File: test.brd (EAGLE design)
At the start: 101.6 x 53.3 mm, 60 parts, among them IC2 ATMEGA1280-16AU, IC4 MC33269D-5.0, IC6 FT232RL, IC7 LM358D, Q2 16MHz, T1 NDT2955, X2 DC21MMX

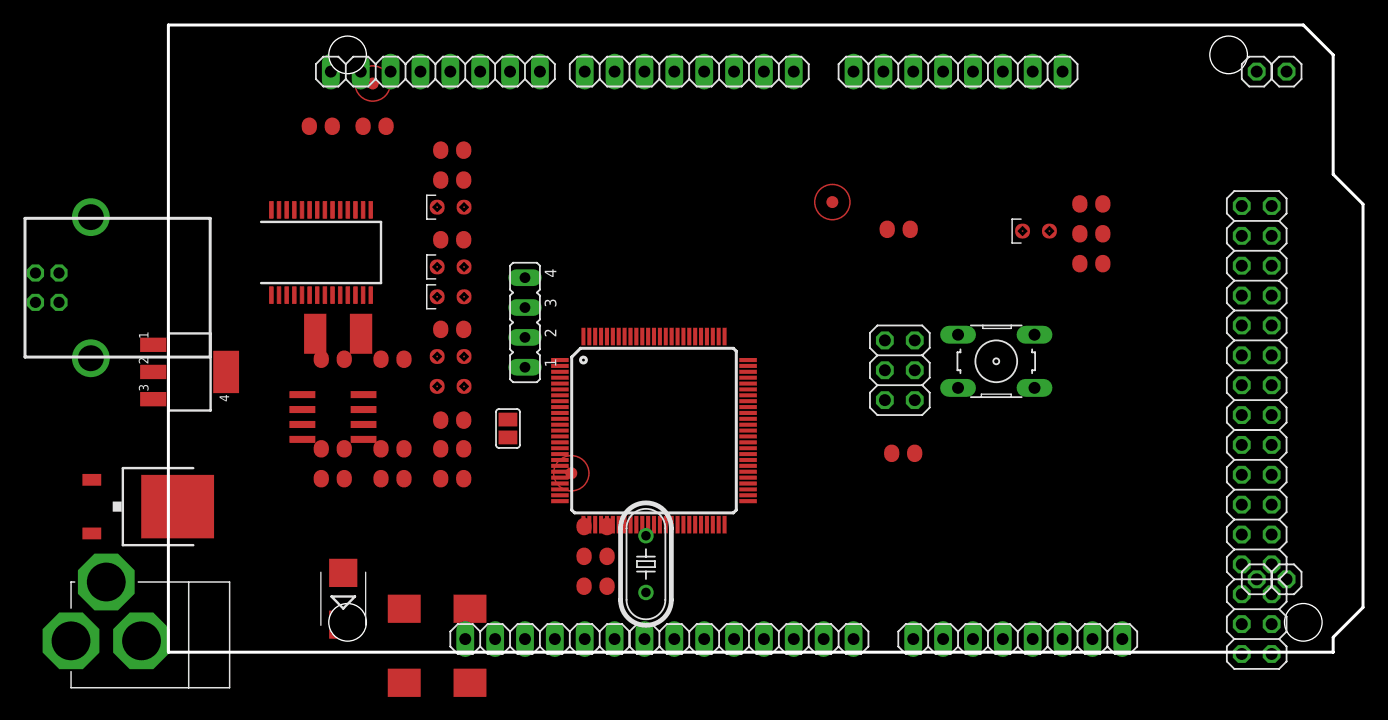
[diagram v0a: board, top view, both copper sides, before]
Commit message: test output
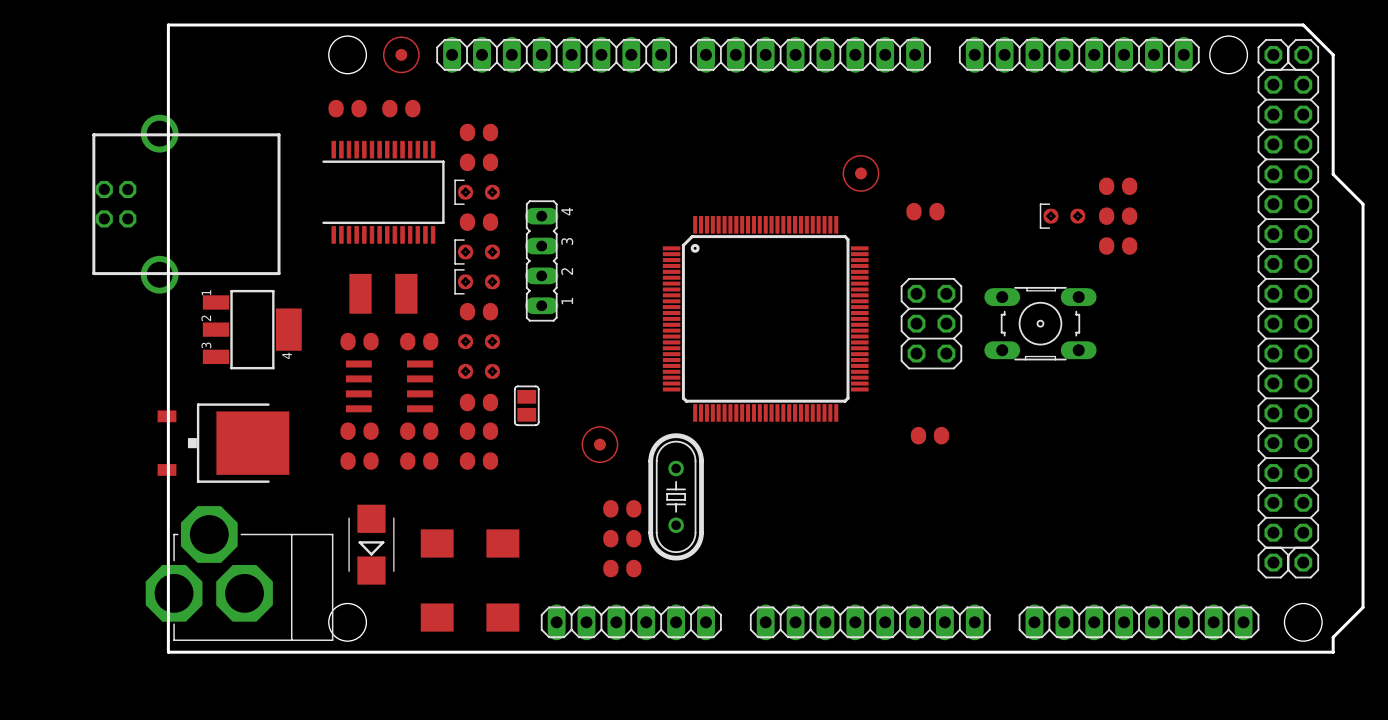
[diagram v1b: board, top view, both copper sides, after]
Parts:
- moved IC2 13.4 mm to (50.8, 28.3)
- moved JP2 10.7 mm to (95.2, 19.1)
- moved JP1 10.7 mm to (95.2, 39.4)
- moved PWMH 10.4 mm to (33.0, 50.8)
- moved ADCH 10.4 mm to (82.5, 2.54)
- moved ADCL 10.4 mm to (59.7, 2.54)
- moved COMMUNICATION 10.4 mm to (77.5, 50.8)
- moved PWML 10.4 mm to (54.6, 50.8)
- moved X2 9.65 mm to (6.83, 4.93)
- moved X4 9.20 mm to (-0.74, 38.1)
- moved IC4 8.37 mm to (4.68, 17.8)
- moved POWER 7.90 mm to (39.4, 2.54)
- moved IC6 7.37 mm to (18.3, 39.1)
- moved T1 6.44 mm to (7.15, 27.4)
- moved Q2 6.26 mm to (43.2, 13.2)
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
